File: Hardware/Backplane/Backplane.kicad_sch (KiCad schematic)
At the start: 3 parts

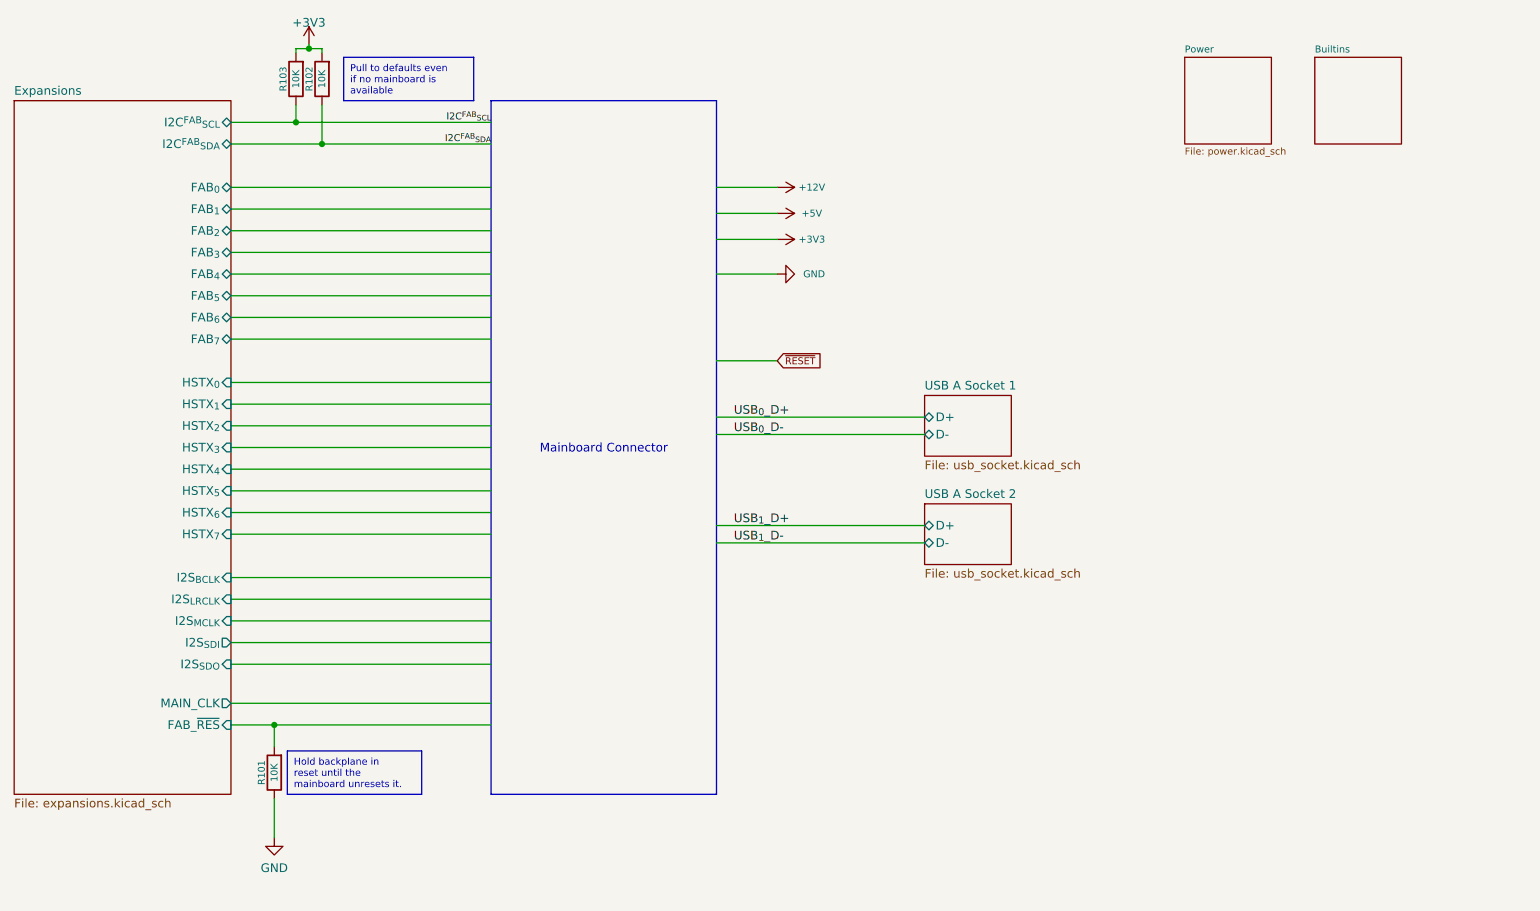
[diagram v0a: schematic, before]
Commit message: Adjusts to review comments
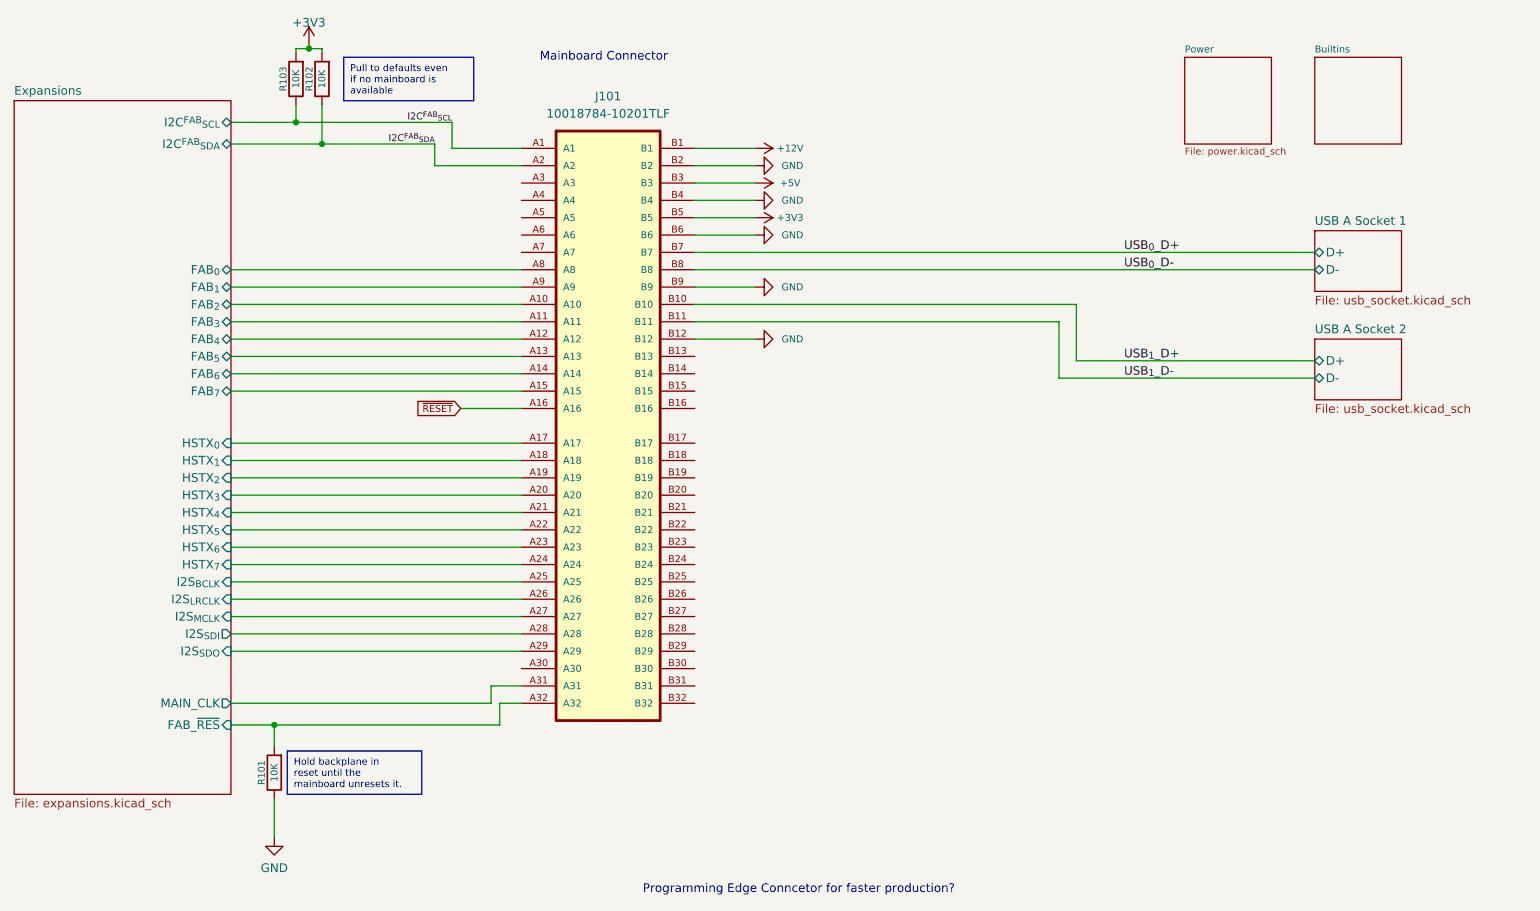
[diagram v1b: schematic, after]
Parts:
- added J101: 10018784-10201TLF, Home Computer:CONN_10018784-10201TLF, symbol Home Computer:10018784-10201TLF
- R101, R102, R103: Digikey Part No (none) -> 311-10.0KHRCT-ND
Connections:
- net +12V: now also J101.B1
- net +3V3: now also J101.B5
- net +5V: now also J101.B3
- net Expansions/FAB_{0}: now also J101.A8
- net Expansions/FAB_{1}: now also J101.A9
- net Expansions/FAB_{2}: now also J101.A10
- net Expansions/FAB_{3}: now also J101.A11
- net Expansions/FAB_{4}: now also J101.A12
- net Expansions/FAB_{5}: now also J101.A13
- net Expansions/FAB_{6}: now also J101.A14
- net Expansions/FAB_{7}: now also J101.A15
- net Expansions/FAB_~{RES}: now also J101.A32
- net Expansions/HSTX_{0}: now also J101.A17
- net Expansions/HSTX_{1}: now also J101.A18
- net Expansions/HSTX_{2}: now also J101.A19
- net Expansions/HSTX_{3}: now also J101.A20
- net Expansions/HSTX_{4}: now also J101.A21
- net Expansions/HSTX_{5}: now also J101.A22
- net Expansions/HSTX_{6}: now also J101.A23
- net Expansions/HSTX_{7}: now also J101.A24
- net Expansions/I2S_{BCLK}: now also J101.A25
- net Expansions/I2S_{LRCLK}: now also J101.A26
- net Expansions/I2S_{MCLK}: now also J101.A27
- net Expansions/I2S_{SDI}: now also J101.A28
- net Expansions/I2S_{SDO}: now also J101.A29
- net Expansions/MAIN_CLK: now also J101.A31
- net GND: now also J101.B12, J101.B2, J101.B4, J101.B6, J101.B9
- net I2C^{FAB}_{SCL}: now also J101.A1
- net I2C^{FAB}_{SDA}: now also J101.A2
- net USB_{0}_D+: now also J101.B7
- net USB_{0}_D-: now also J101.B8
- net USB_{1}_D+: now also J101.B10
- net USB_{1}_D-: now also J101.B11
- net ~{RESET}: now also J101.A16
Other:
- note added: "Mainboard Connector"
- note added: "Programming Edge Conncetor for faster production?"
